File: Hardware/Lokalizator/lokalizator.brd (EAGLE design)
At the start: 94.9 x 74.9 mm, 19 parts, among them IC1 ATMEGA328PROUND, X1 1268-120, X2 1268-120, X3 1297-25, X4 1297-25

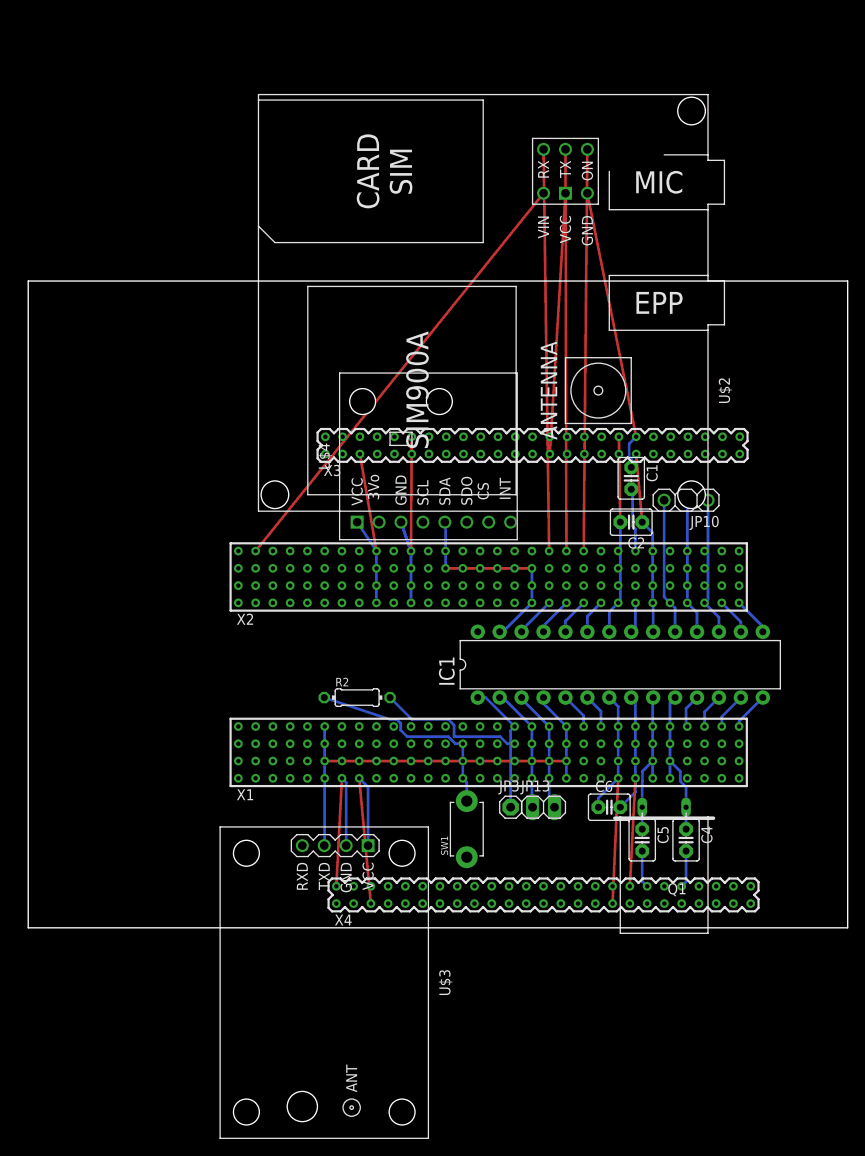
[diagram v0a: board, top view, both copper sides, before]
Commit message: Add files via upload
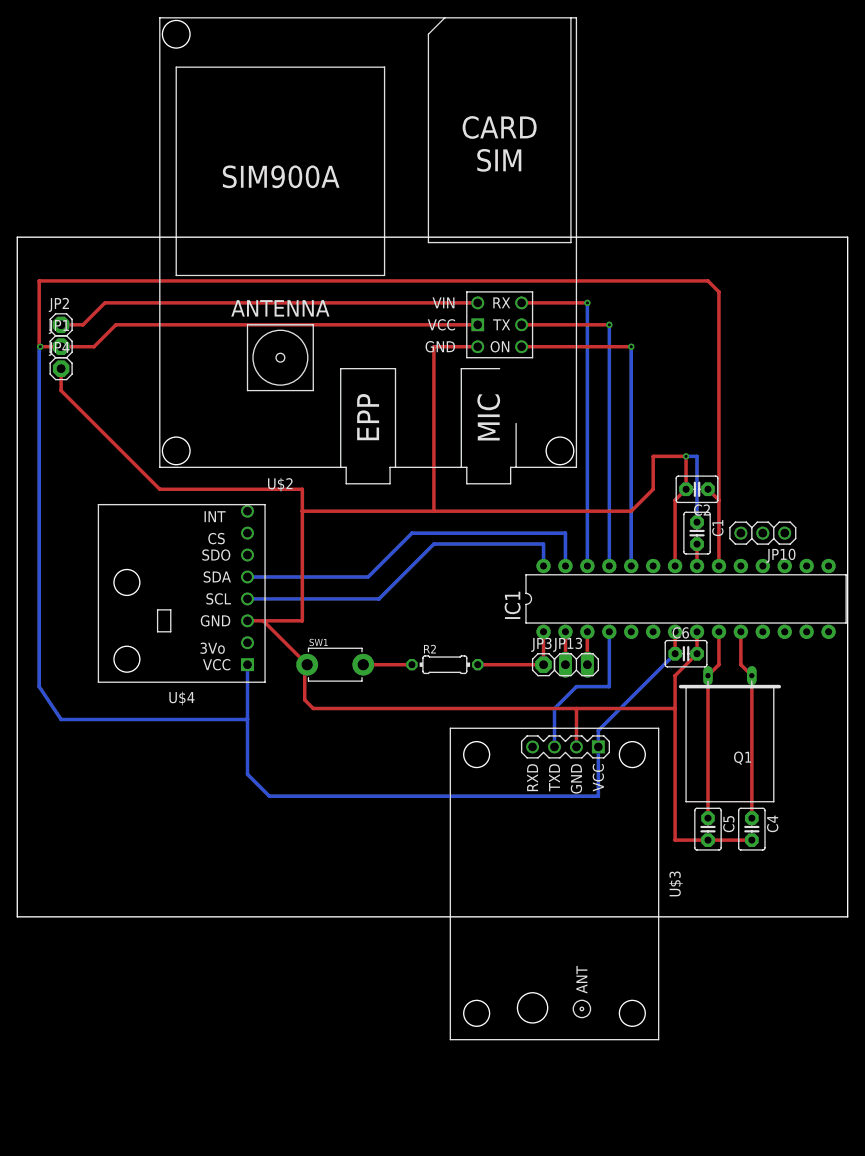
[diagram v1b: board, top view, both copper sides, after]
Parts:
- removed X1, X2: 1268-120, con-commcon:1268-120
- removed X3, X4: 1297-25, con-commcon:1297-25
- added JP1, JP2, JP4: (no value), adafruit:1X01
- moved U$4 31.8 mm to (19.1, 34.3), turned to 180 degrees
- moved U$3 29.0 mm to (62.2, 3.81)
- moved SW1 24.4 mm to (36.8, 29.2), turned to 0 degrees
- moved C6 19.9 mm to (77.5, 30.5)
- moved Q1 17.0 mm to (82.5, 20.3)
- moved JP3 16.9 mm to (61.0, 29.2)
- moved JP13 16.9 mm to (64.8, 29.2)
- moved U$2 14.8 mm to (40.6, 78.7), turned to 180 degrees
- moved R2 10.9 mm to (49.5, 29.2)
- moved IC1 10.8 mm to (77.5, 36.8)
- moved C1 9.92 mm to (78.7, 44.5)
- moved JP10 9.67 mm to (86.4, 44.5)
- moved C2 8.52 mm to (78.7, 49.5)
- moved C4 7.73 mm to (85.1, 10.2)
- moved C5 7.73 mm to (80.0, 10.2)
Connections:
- removed net N$1: R2.1, SW1.P$2, X1.A14, X1.B14, X1.C14, X1.D14
- removed net N$10: IC1.14, X1.A30, X1.B30, X1.C30, X1.D30
- removed net N$19: IC1.15, X2.A30, X2.B30, X2.C30, X2.D30
- removed net N$20: IC1.16, X2.A29, X2.B29, X2.C29, X2.D29
- removed net N$23: IC1.11, X1.A27, X1.B27, X1.C27, X1.D27
- removed net N$24: IC1.23, X2.A22, X2.B22, X2.C22, X2.D22
- removed net N$25: IC1.5, X1.A21, X1.B21, X1.C21, X1.D21
- removed net N$26: IC1.27, U$4.4, X2.A13, X2.A18, X2.B13, X2.B18, X2.C13, X2.C18, X2.D13, X2.D18
- removed net N$27: IC1.6, X1.A22, X1.B22, X1.C22, X1.D22
- removed net N$28: X1.A15, X1.B15, X1.C15, X1.D15
- removed net N$29: X1.A13, X1.B13, X1.C13, X1.D13
- removed net N$30: X1.A12, X1.B12, X1.C12, X1.D12
- removed net N$31: X1.A11, X1.B11, X1.C11, X1.D11
- removed net N$32: X1.A10, X1.B10, X1.C10, X1.D10
- removed net N$33: X1.A9, X1.B9, X1.C9, X1.D9
- removed net N$37: X1.A5, X1.B5, X1.C5, X1.D5
- removed net N$38: X1.A4, X1.B4, X1.C4, X1.D4
- removed net N$39: X1.A3, X1.B3, X1.C3, X1.D3
- removed net N$40: X1.A2, X1.B2, X1.C2, X1.D2
- removed net N$41: X1.A1, X1.B1, X1.C1, X1.D1
- removed net N$42: X2.A16, X2.B16, X2.C16, X2.D16
- removed net N$43: X2.A15, X2.B15, X2.C15, X2.D15
- removed net N$44: X2.A14, X2.B14, X2.C14, X2.D14
- removed net N$48: X2.A10, X2.B10, X2.C10, X2.D10
- removed net N$50: X2.A8, X2.B8, X2.C8, X2.D8
- removed net N$51: X2.A7, X2.B7, X2.C7, X2.D7
- removed net N$52: X2.A6, X2.B6, X2.C6, X2.D6
- removed net N$53: X2.A5, X2.B5, X2.C5, X2.D5
- removed net N$54: X2.A4, X2.B4, X2.C4, X2.D4
- removed net N$55: X2.A3, X2.B3, X2.C3, X2.D3
- removed net N$57: X2.A1, X2.B1, X2.C1, X2.D1
- removed net N$7: C4.1, IC1.10, Q1.1, X1.A26, X1.B26, X1.C26, X1.D26
- net GND: now also JP4.1; no longer X1.A24, X1.A7, X1.B24, X1.B7, X1.C24, X1.C7, X1.D24, X1.D7, X2.A11, X2.A23, X2.B11, X2.B23, X2.C11, X2.C23, X2.D11, X2.D23, X3.B1, X3.B10, X3.B11, X3.B12, X3.B13, X3.B14, X3.B15, X3.B16, X3.B17, X3.B18, X3.B19, X3.B2, X3.B20, X3.B21, X3.B22, X3.B23, X3.B24, X3.B25, X3.B3, X3.B4, X3.B5, X3.B6, X3.B7, X3.B8, X3.B9, X4.B1, X4.B10, X4.B11, X4.B12, X4.B13, X4.B14, X4.B15, X4.B16, X4.B17, X4.B18, X4.B19, X4.B2, X4.B20, X4.B21, X4.B22, X4.B23, X4.B24, X4.B25, X4.B3, X4.B4, X4.B5, X4.B6, X4.B7, X4.B8, X4.B9
- net N$11: now also C4.1, IC1.10, Q1.1; no longer IC1.28, U$4.5, X2.A12, X2.A17, X2.B12, X2.B17, X2.C12, X2.C17, X2.D12, X2.D17
- net N$12: now also IC1.27, U$4.4; no longer X1.A16, X1.B16, X1.C16, X1.D16
- net N$13: no longer X1.A20, X1.A6, X1.B20, X1.B6, X1.C20, X1.C6, X1.D20, X1.D6
- net N$14: no longer X2.A21, X2.B21, X2.C21, X2.D21
- net N$15: no longer X1.A18, X1.B18, X1.C18, X1.D18
- net N$16: no longer X1.A19, X1.B19, X1.C19, X1.D19
- net N$17: no longer X2.A20, X2.B20, X2.C20, X2.D20
- net N$18: no longer X2.A19, X2.B19, X2.C19, X2.D19
- net N$2: no longer X1.A17, X1.B17, X1.C17, X1.D17
- net N$21: now also IC1.28, U$4.5; no longer IC1.13, X1.A29, X1.B29, X1.C29, X1.D29
- net N$22: now also R2.1, SW1.P$2; no longer IC1.12, X1.A28, X1.B28, X1.C28, X1.D28
- net N$3: no longer X2.A24, X2.B24, X2.C24, X2.D24
- net N$5: no longer X2.A26, X2.B26, X2.C26, X2.D26
- net N$6: no longer X1.A25, X1.B25, X1.C25, X1.D25
- net N$8: no longer X2.A27, X2.B27, X2.C27, X2.D27
- net N$9: no longer X2.A28, X2.B28, X2.C28, X2.D28
- net VCC: now also JP1.1, JP2.1; no longer X1.A23, X1.A8, X1.B23, X1.B8, X1.C23, X1.C8, X1.D23, X1.D8, X2.A2, X2.A25, X2.A9, X2.B2, X2.B25, X2.B9, X2.C2, X2.C25, X2.C9, X2.D2, X2.D25, X2.D9, X3.A1, X3.A10, X3.A11, X3.A12, X3.A13, X3.A14, X3.A15, X3.A16, X3.A17, X3.A18, X3.A19, X3.A2, X3.A20, X3.A21, X3.A22, X3.A23, X3.A24, X3.A25, X3.A3, X3.A4, X3.A5, X3.A6, X3.A7, X3.A8, X3.A9, X4.A1, X4.A10, X4.A11, X4.A12, X4.A13, X4.A14, X4.A15, X4.A16, X4.A17, X4.A18, X4.A19, X4.A2, X4.A20, X4.A21, X4.A22, X4.A23, X4.A24, X4.A25, X4.A3, X4.A4, X4.A5, X4.A6, X4.A7, X4.A8, X4.A9
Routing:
- net VCC: track 177.4 -> 364.4 mm, vias 0 -> 1
- net GND: track 138.0 -> 245.7 mm, vias 0 -> 1
- net N$12: track 0.00 -> 42.7 mm
- net N$21: track 4.27 -> 39.5 mm
- net N$13: track 52.3 -> 18.2 mm
- net N$1: track 24.9 -> 0.00 mm
- net N$26: track 24.5 -> 0.00 mm
- net N$11: track 0.00 -> 22.1 mm
- net N$2: track 32.6 -> 11.4 mm
- net N$7: track 18.3 -> 0.00 mm
- net N$9: track 16.1 -> 0.00 mm
- net N$5: track 15.8 -> 0.00 mm
- net N$8: track 15.8 -> 0.00 mm
- net N$18: track 51.2 -> 38.1 mm, vias 0 -> 1
- net N$17: track 51.0 -> 38.1 mm, vias 0 -> 1
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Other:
- board size 94.9 x 74.9 mm -> 96.2 x 78.7 mm
